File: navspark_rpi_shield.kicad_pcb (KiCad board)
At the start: 2 copper layers, 45 x 42 mm, 7 parts, among them P1 CONN_02X13, P2 CONN_01X13, P3 CONN_01X12

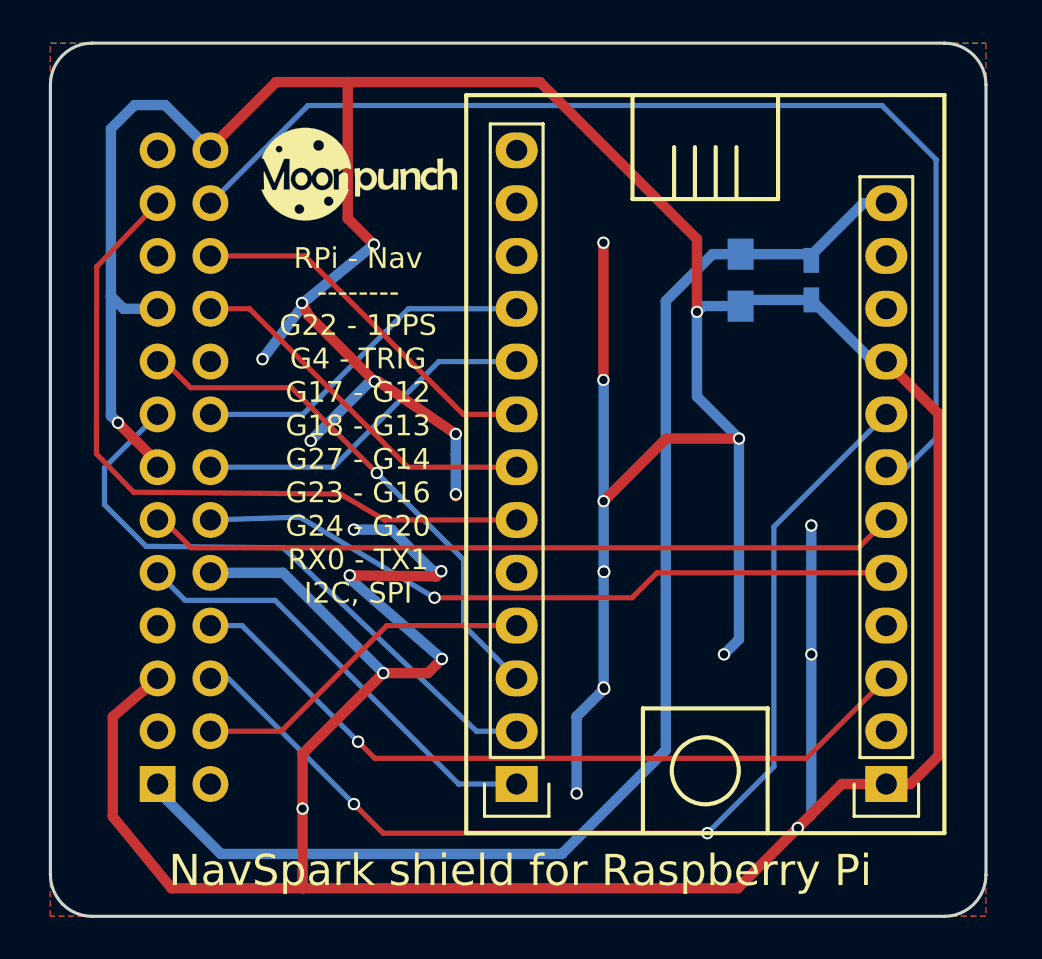
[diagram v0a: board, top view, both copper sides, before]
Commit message: add v2 of the board
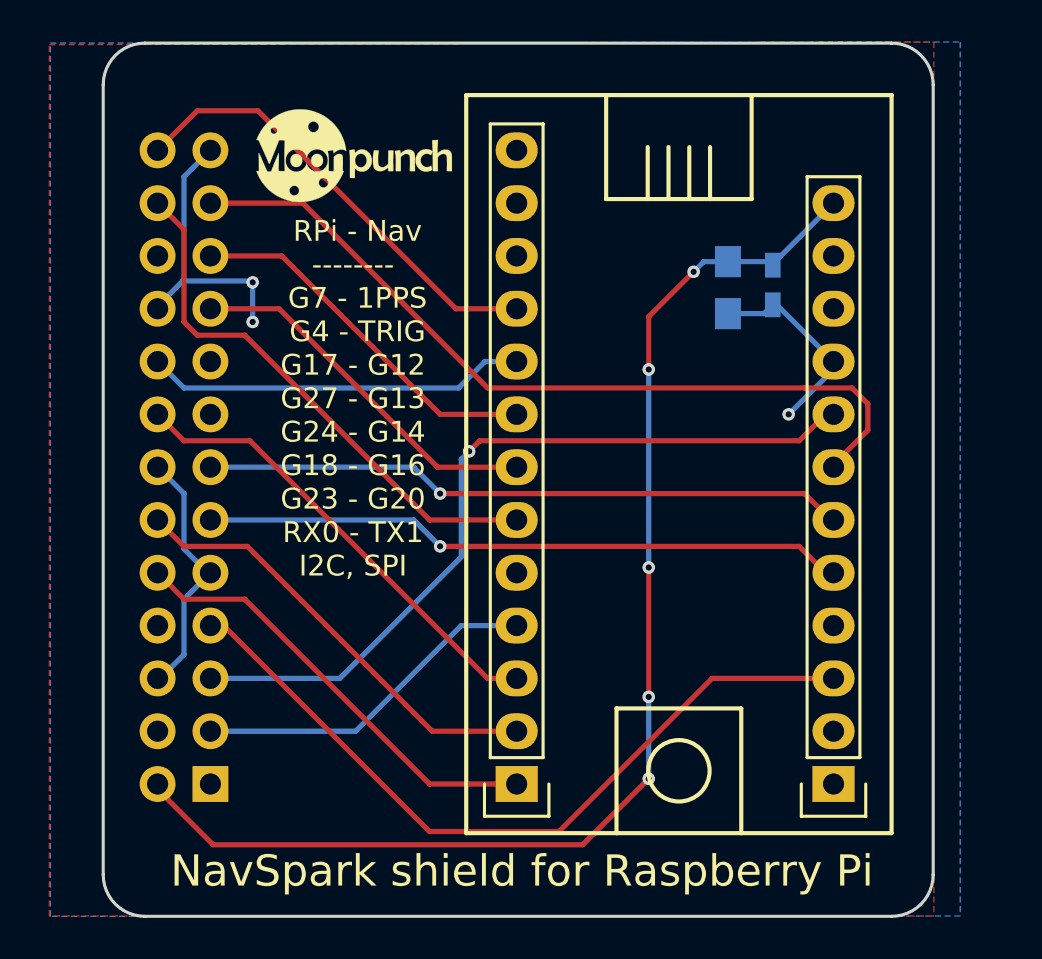
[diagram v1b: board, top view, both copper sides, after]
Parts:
- P1: value CONN_02X13 -> RPI_02X13; footprint Pin_Headers:Pin_Header_Straight_2x13 -> Socket_Strips:Socket_Strip_Straight_2x13
- P2: value CONN_01X13 -> NAV_01X13; footprint Pin_Headers:Pin_Header_Straight_1x13 -> Socket_Strips:Socket_Strip_Straight_1x13
- P3: value CONN_01X12 -> NAV_01X12; footprint Pin_Headers:Pin_Header_Straight_1x12 -> Socket_Strips:Socket_Strip_Straight_1x12
- moved P1 2.54 mm to (107.7, 135.6), turned to 90 degrees
- moved P3 2.54 mm to (137.7, 135.6), turned to 90 degrees
- moved C2 1.87 mm to (134.7, 111.6)
- moved G*** 1.47 mm to (130.3, 134.0)
- moved G*** 0.92 mm to (114.6, 105.4)
- moved C1 0.71 mm to (132.6, 111.8)
- turned P2 to 90 degrees
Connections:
- P1 pad 1: VCC -> Net-(P1-Pad1)
- P1 pad 10: GND -> /N_TXD1
- P1 pad 11: /GPIO13 -> /GPIO12
- P1 pad 12: /GPIO12 -> /GPIO16
- P1 pad 13: GND -> /GPIO13
- P1 pad 14: /GPIO14 -> GND
- P1 pad 15: /GPIO16 -> Net-(P1-Pad15)
- P1 pad 16: /1PPS -> /GPIO20
- P1 pad 17: /GPIO20 -> Net-(P1-Pad17)
- P1 pad 18: Net-(P1-Pad18) -> /GPIO14
- P1 pad 19: GND -> /SPI_MOSI
- P1 pad 2: Net-(P1-Pad2) -> VCC
- P1 pad 20: /SPI_MOSI -> GND
- P1 pad 21: Net-(P1-Pad21) -> /SPI_MISO
- P1 pad 22: /SPI_MISO -> Net-(P1-Pad22)
- P1 pad 23: /SPI_CSN0 -> /SPI_SCK
- P1 pad 24: /SPI_SCK -> /SPI_CSN0
- P1 pad 25: Net-(P1-Pad25) -> GND
- P1 pad 26: GND -> /1PPS
- P1 pad 3: Net-(P1-Pad3) -> /I2C_SDA
- P1 pad 4: /I2C_SDA -> Net-(P1-Pad4)
- P1 pad 5: GND -> /I2C_SCL
- P1 pad 6: /I2C_SCL -> GND
- P1 pad 7: Net-(P1-Pad7) -> /TRIG
- P1 pad 8: /TRIG -> Net-(P1-Pad8)
- P1 pad 9: /N_TXD1 -> GND
- P3 pad 1: GND -> Net-(P3-Pad1)
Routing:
- net GND: track 281.3 -> 36.2 mm, vias 28 -> 3
- net /SPI_SCK: track 54.3 -> 39.7 mm
- net /I2C_SCL: track 50.7 -> 38.0 mm, vias 2 -> 1
- net /SPI_CSN0: track 34.6 -> 26.2 mm
- net /GPIO16: track 29.6 -> 21.8 mm
- net /1PPS: track 16.8 -> 22.0 mm
- net /GPIO13: track 36.2 -> 31.0 mm, vias 0 -> 1
- net /GPIO12: track 34.1 -> 31.0 mm
- net /GPIO20: track 25.4 -> 22.5 mm, vias 1 -> 0
- net VCC: track 62.6 -> 60.2 mm, vias 0 -> 5
- net /GPIO14: track 16.8 -> 18.7 mm
- net /TRIG: track 36.7 -> 37.1 mm, vias 1 -> 0
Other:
- board size 45 x 42 mm -> 39.9 x 42 mm
- net class Default: clearance 0.2 -> 0.2032; via_drill 0.4 -> 0.3
- net class Power: clearance 0.2 -> 0.2032; trace_width 0.5 -> 0.25; via_drill 0.4 -> 0.3
- rule trace_clearance: 0.2 -> 0.2032
- board text added: "RPi - Nav -------- G7 - 1PPS G4 - TRIG G17 - G12 G27 - G13 G24 - G14 G18 - G16 G23 - G20 RX0 - TX1 I2C, SPI"
- board text added: "v2, 2016-01-15"
- board text removed: "RPi - Nav -------- G22 - 1PPS G4 - TRIG G17 - G12 G18 - G13 G27 - G14 G23 - G16 G24 - G20 RX0 - TX1 I2C, SPI"
- board text removed: "v1, 2015 Dec 21"
